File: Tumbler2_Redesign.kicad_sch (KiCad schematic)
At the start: 4 parts

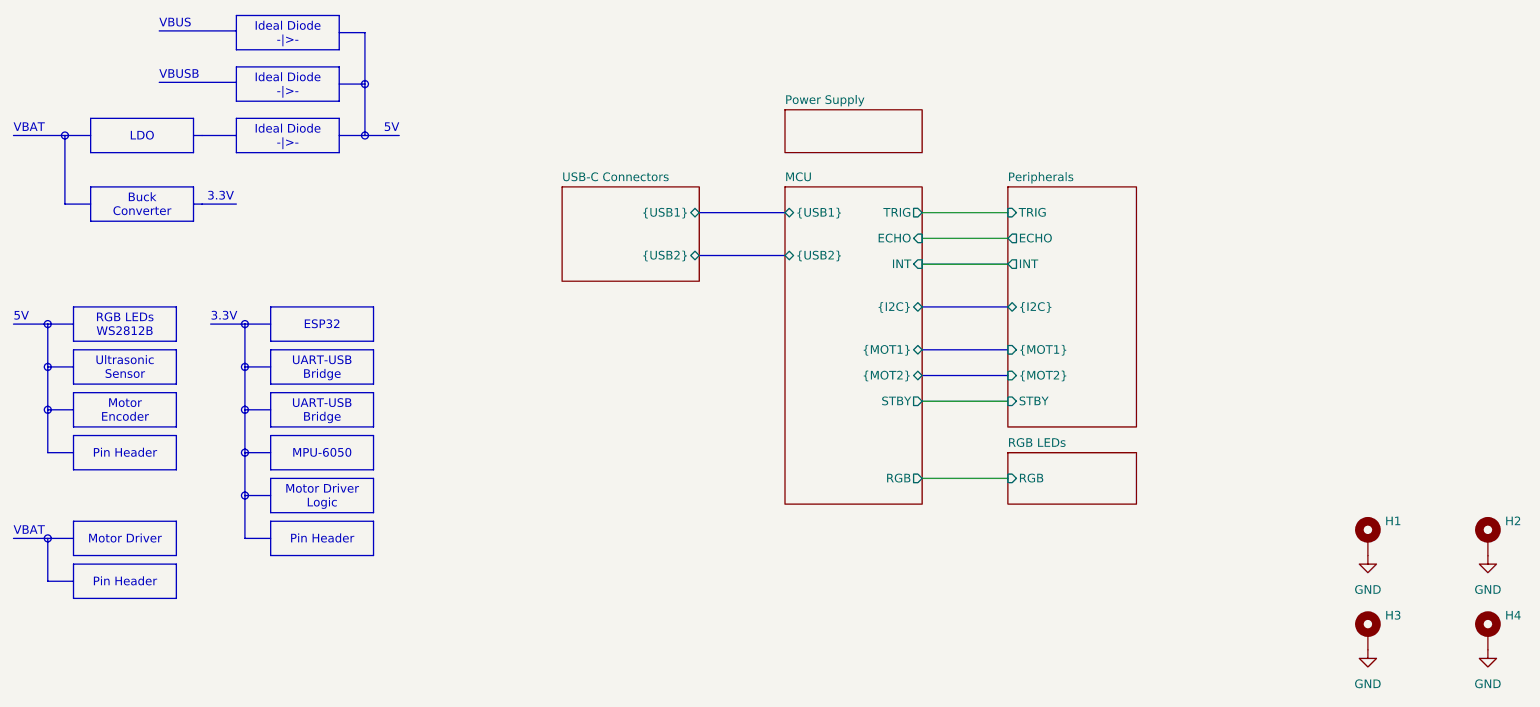
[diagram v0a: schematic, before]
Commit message: Sketch out component placement
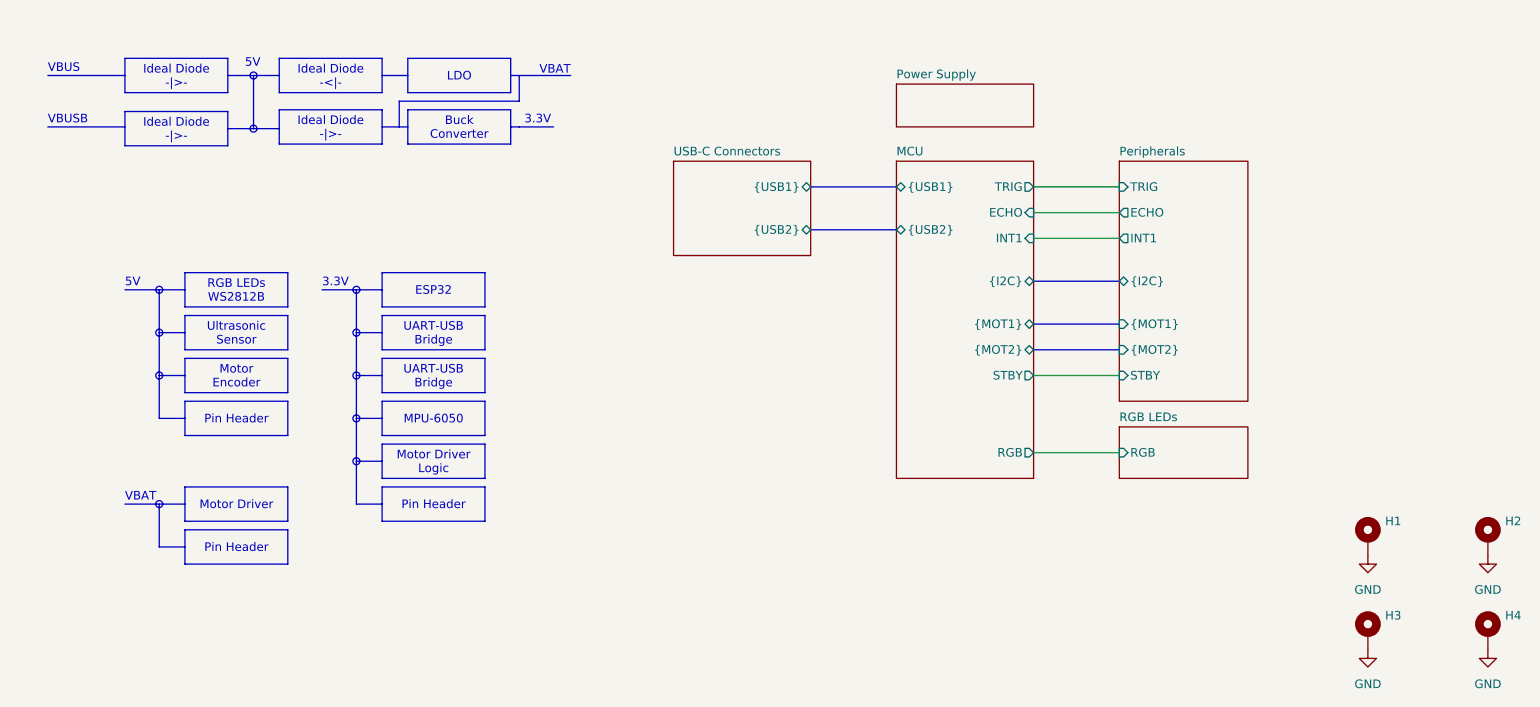
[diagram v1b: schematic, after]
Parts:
- H1, H2, H3, H4: footprint MountingHole:MountingHole_3mm_Pad -> MountingHole:MountingHole_3mm_Pad_Via
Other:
- sheet MCU ports: added INT1; removed INT
- sheet Peripherals ports: added INT1; removed INT
